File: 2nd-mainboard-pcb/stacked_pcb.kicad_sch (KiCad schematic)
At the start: 7 parts, among them J17 Steckverbinder_Male_1, J18 Steckverbinder_Male_2, J19 Steckverbinder_Female_2

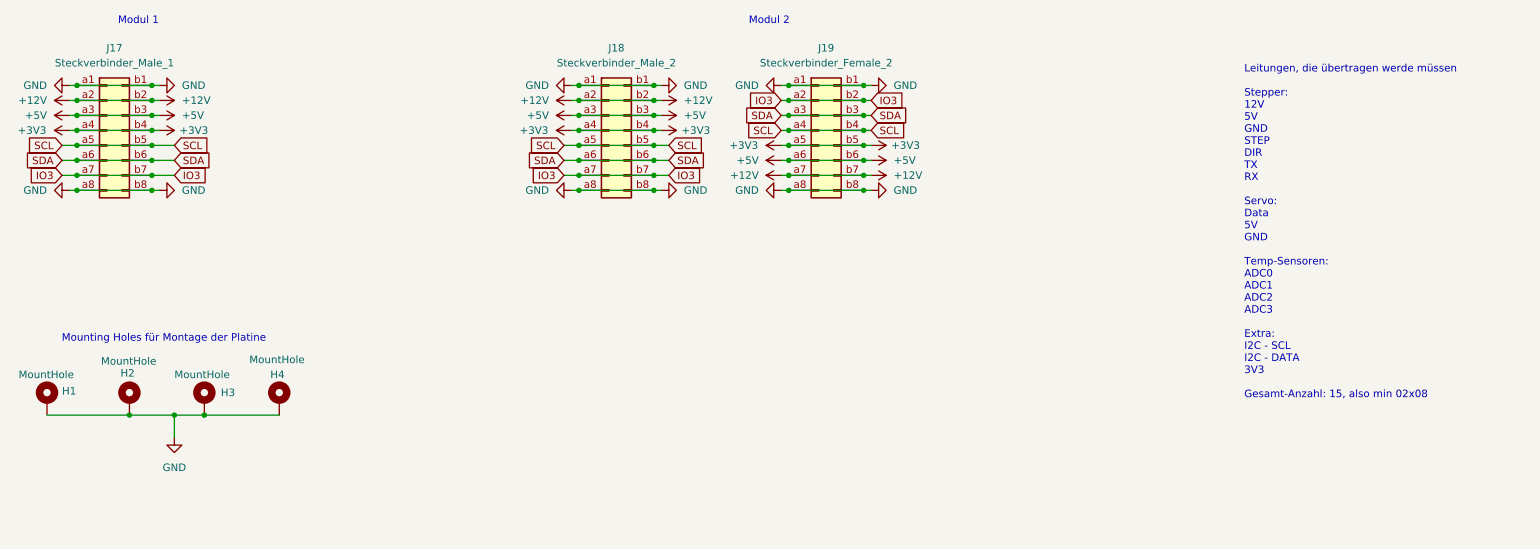
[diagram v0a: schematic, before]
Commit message: finished stacked design, annotaded
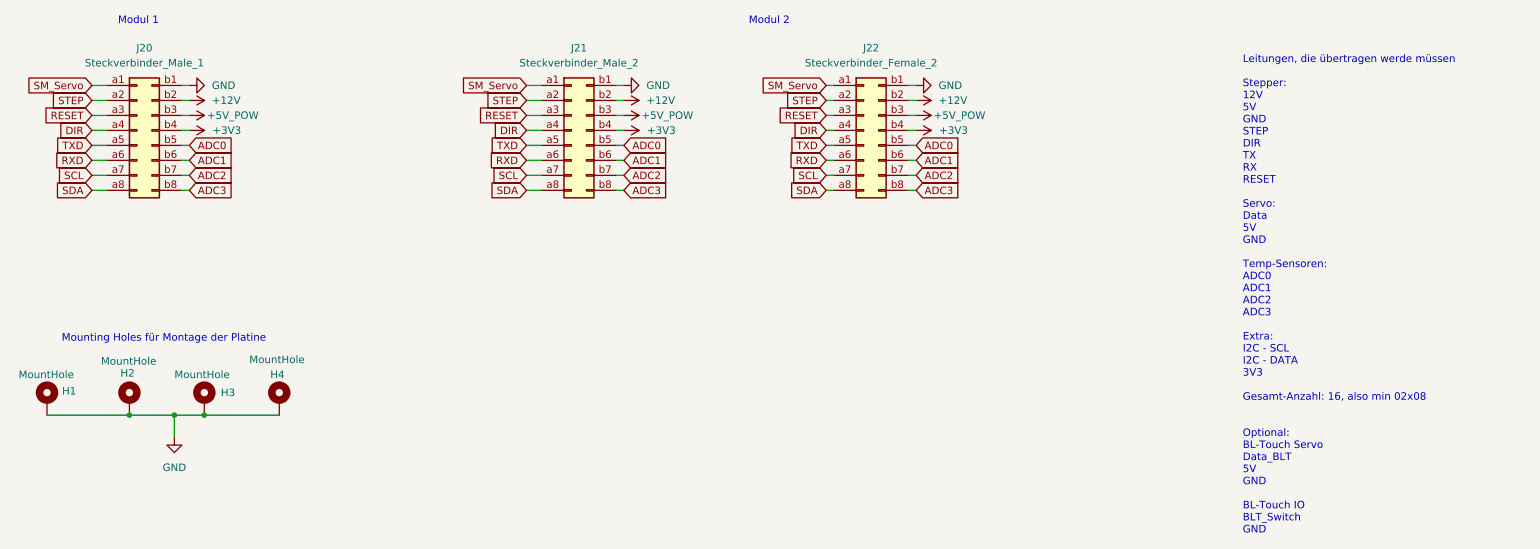
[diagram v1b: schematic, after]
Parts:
- removed J18: Steckverbinder_Male_2, CustomFotLibByJan:BF100-16-A-D-1-0640-L-C, symbol Connector_Generic:Conn_02x08_Row_Letter_First
- added J21: Steckverbinder_Male_2, CustomFotLibByJan:BF100-16-A-D-1-0640-L-C, symbol Connector_Generic:Conn_02x08_Row_Letter_First
- renumbered J17 to J20, J19 to J22
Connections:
- net +12V: now also J22.b2 (Pin_b2), J21.b2 (Pin_b2); no longer J20.a2 (Pin_a2), J22.a7 (Pin_a7), J22.b7 (Pin_b7)
- net +3V3: now also J22.b4 (Pin_b4), J21.b4 (Pin_b4); no longer J20.a4 (Pin_a4), J22.a5 (Pin_a5), J22.b5 (Pin_b5)
- net GND: now also J21.b1 (Pin_b1); no longer J20.a1 (Pin_a1), J20.a8 (Pin_a8), J20.b8 (Pin_b8), J22.a1 (Pin_a1), J22.a8 (Pin_a8), J22.b8 (Pin_b8)
- net SCL: now also J20.a7 (Pin_a7), J22.a7 (Pin_a7), J21.a7 (Pin_a7); no longer J20.a5 (Pin_a5), J20.b5 (Pin_b5), J22.a4 (Pin_a4), J22.b4 (Pin_b4)
- net SDA: now also J20.a8 (Pin_a8), J22.a8 (Pin_a8), J21.a8 (Pin_a8); no longer J20.a6 (Pin_a6), J20.b6 (Pin_b6), J22.a3 (Pin_a3), J22.b3 (Pin_b3)
- removed net +5V: J20.a3 (Pin_a3), J20.b3 (Pin_b3), J22.a6 (Pin_a6), J22.b6 (Pin_b6)
- removed net IO3: J20.a7 (Pin_a7), J20.b7 (Pin_b7), J22.a2 (Pin_a2), J22.b2 (Pin_b2)
- new net +5V_POW: J20.b3 (Pin_b3), J21.b3 (Pin_b3), J22.b3 (Pin_b3)
- new net ADC0: J20.b5 (Pin_b5), J21.b5 (Pin_b5), J22.b5 (Pin_b5)
- new net ADC1: J20.b6 (Pin_b6), J21.b6 (Pin_b6), J22.b6 (Pin_b6)
- new net ADC2: J20.b7 (Pin_b7), J21.b7 (Pin_b7), J22.b7 (Pin_b7)
- new net ADC3: J20.b8 (Pin_b8), J21.b8 (Pin_b8), J22.b8 (Pin_b8)
- new net DIR: J20.a4 (Pin_a4), J21.a4 (Pin_a4), J22.a4 (Pin_a4)
- new net RESET: J20.a3 (Pin_a3), J21.a3 (Pin_a3), J22.a3 (Pin_a3)
- new net RXD: J20.a6 (Pin_a6), J21.a6 (Pin_a6), J22.a6 (Pin_a6)
- new net SM_Servo: J20.a1 (Pin_a1), J21.a1 (Pin_a1), J22.a1 (Pin_a1)
- new net STEP: J20.a2 (Pin_a2), J21.a2 (Pin_a2), J22.a2 (Pin_a2)
- new net TXD: J20.a5 (Pin_a5), J21.a5 (Pin_a5), J22.a5 (Pin_a5)
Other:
- note added: "Leitungen, die übertragen werde müssen Stepper: 12V 5V GND STEP DIR TX RX RESET Servo: Data 5V GND Temp-Sensoren: ADC0 ADC1 ADC2 ADC3 Extra: I2C - SCL I2C - DATA 3V3 Gesamt-Anzahl: 16, also min 02x08 Optional: BL-Touch Servo Data_BLT 5V GND BL-Touch IO BLT_Switch GND"
- note removed: "Leitungen, die übertragen werde müssen Stepper: 12V 5V GND STEP DIR TX RX Servo: Data 5V GND Temp-Sensoren: ADC0 ADC1 ADC2 ADC3 Extra: I2C - SCL I2C - DATA 3V3 Gesamt-Anzahl: 15, also min 02x08"
- moved on the sheet: J20, J22
